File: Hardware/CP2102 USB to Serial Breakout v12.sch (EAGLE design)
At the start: 18 parts, among them U1 CP2102, X1 USBPTH

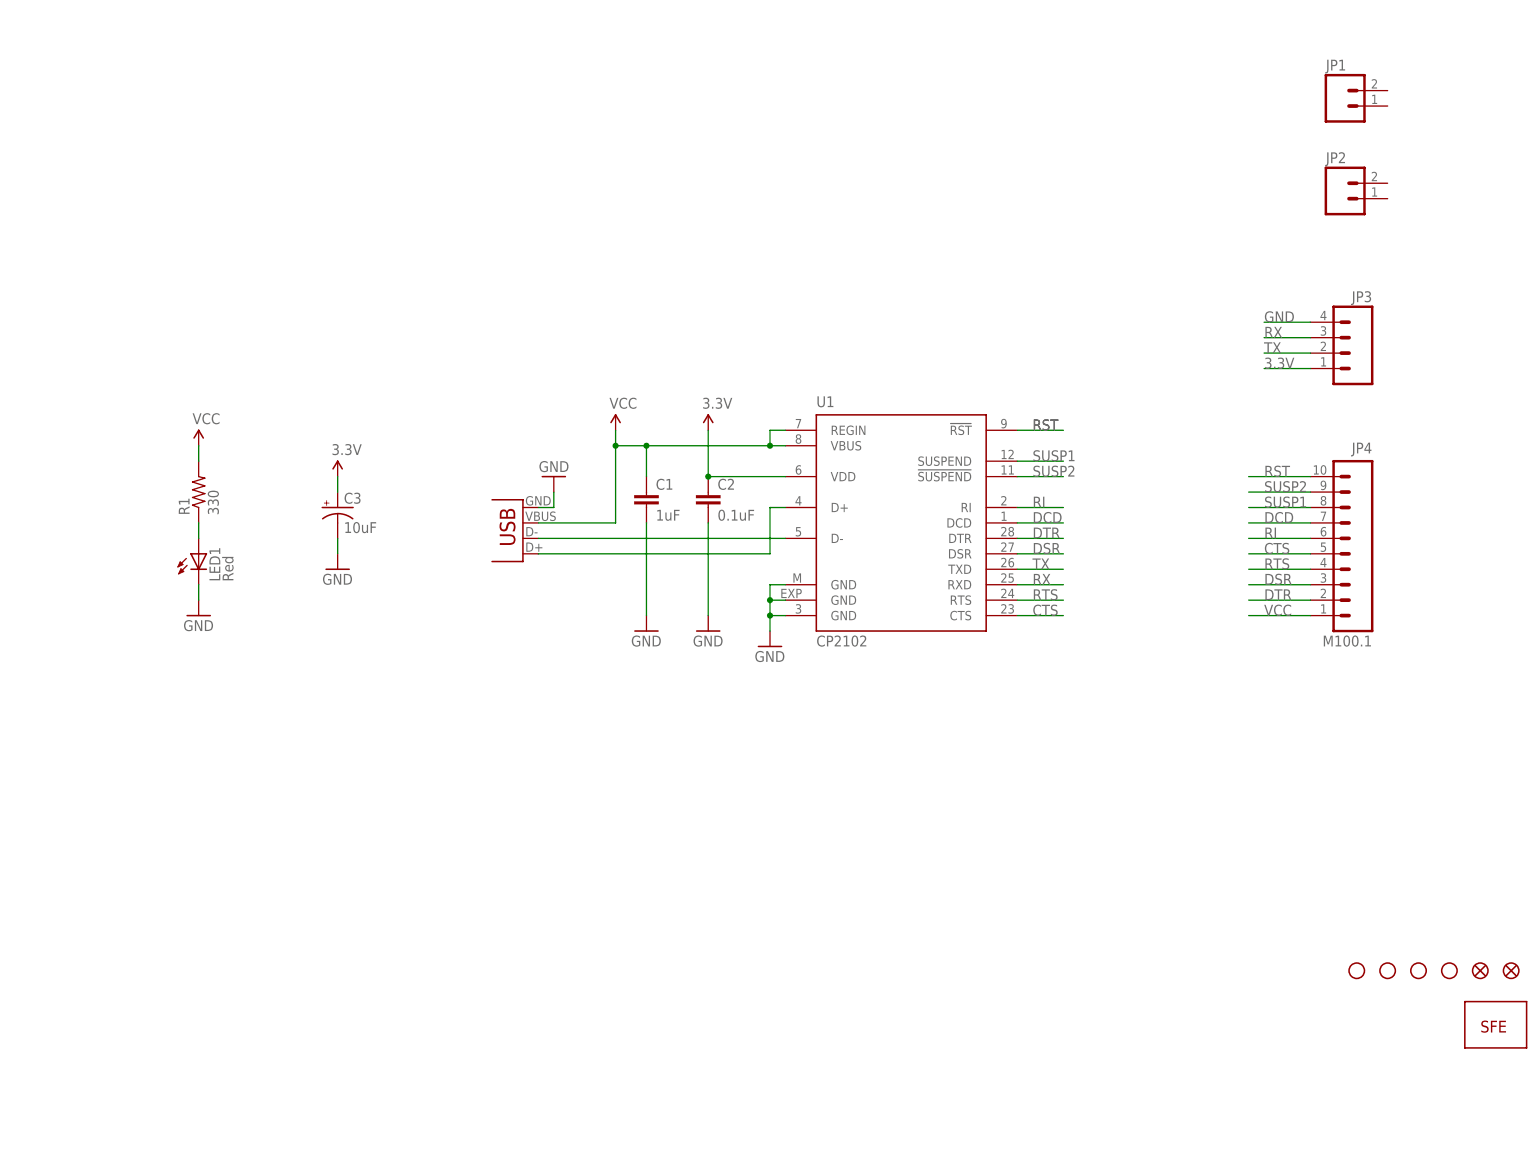
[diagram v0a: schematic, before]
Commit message: Version 1.3 files
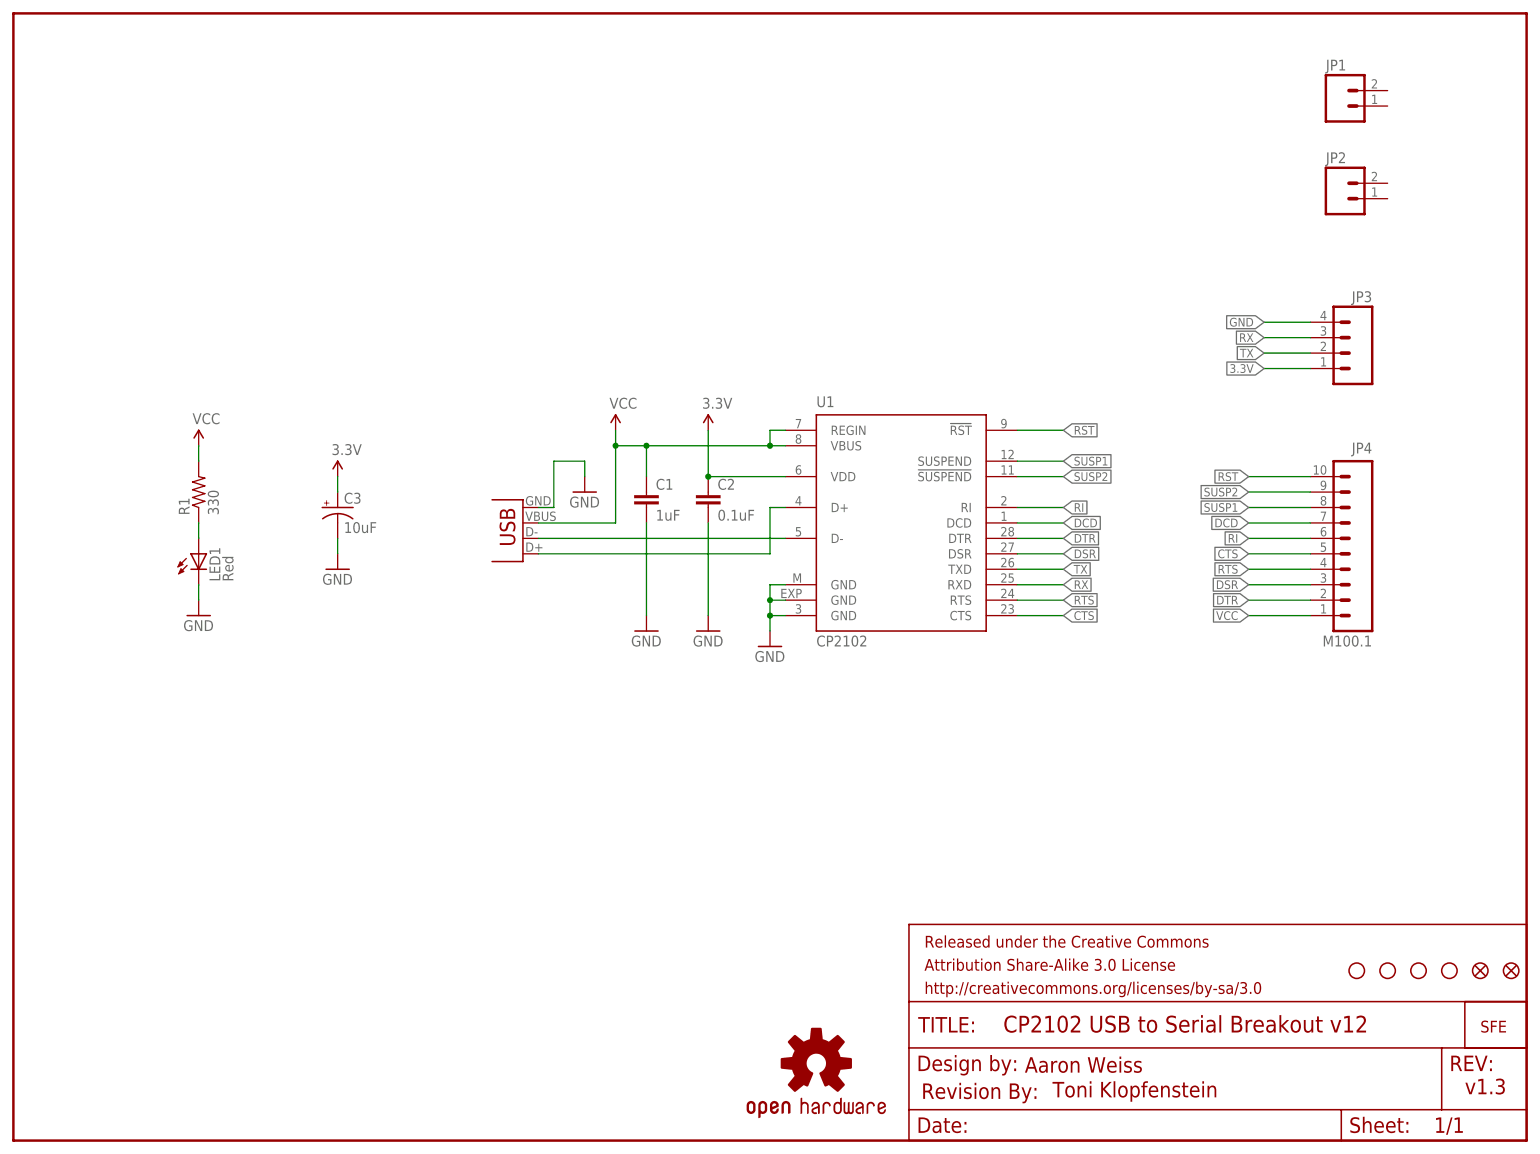
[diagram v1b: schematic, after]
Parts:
- added FRAME1: FRAME-LETTER, SparkFun-Aesthetics:FRAME-LETTER
- added LOGO1: OSHW-LOGOS, SparkFun-Aesthetics:OSHW-LOGOS
- added U$4: REVISION, SparkFun-Aesthetics:REVISION
- C1: device SparkFun:CAP0603 -> SparkFun-Capacitors:1.0UF-16V-10%(0603)
- C2: device SparkFun:CAP0603 -> SparkFun-Capacitors:0.1UF-25V(+80/-20%)(0603)
- R1: device SparkFun:RESISTOR0603 -> SparkFun-Resistors:330OHM1/10W1%(0603)
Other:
- note added: "Aaron Weiss"
- note added: "Toni Klopfenstein"
- note added: "v1.3"
